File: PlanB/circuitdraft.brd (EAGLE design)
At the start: 24 x 43 mm, 23 parts, among them Q1 16 MHz

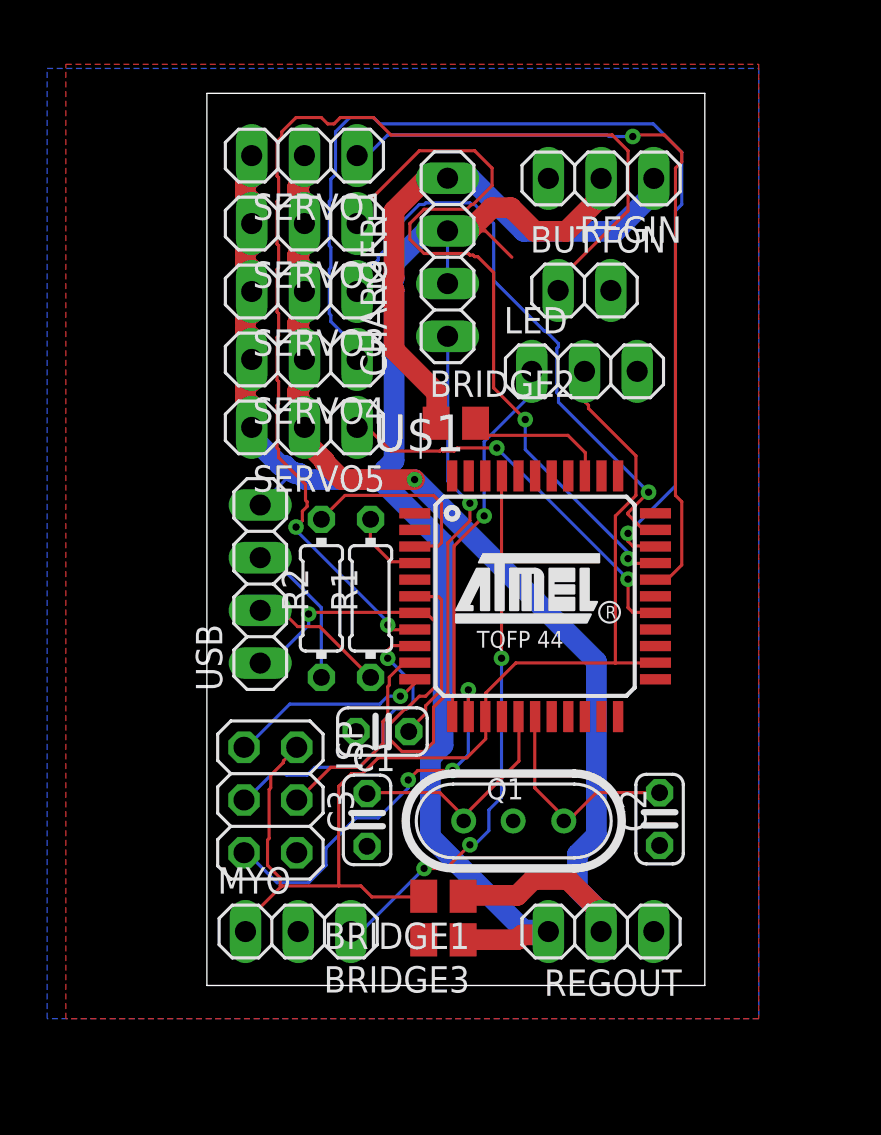
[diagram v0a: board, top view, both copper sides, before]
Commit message: more ajustments
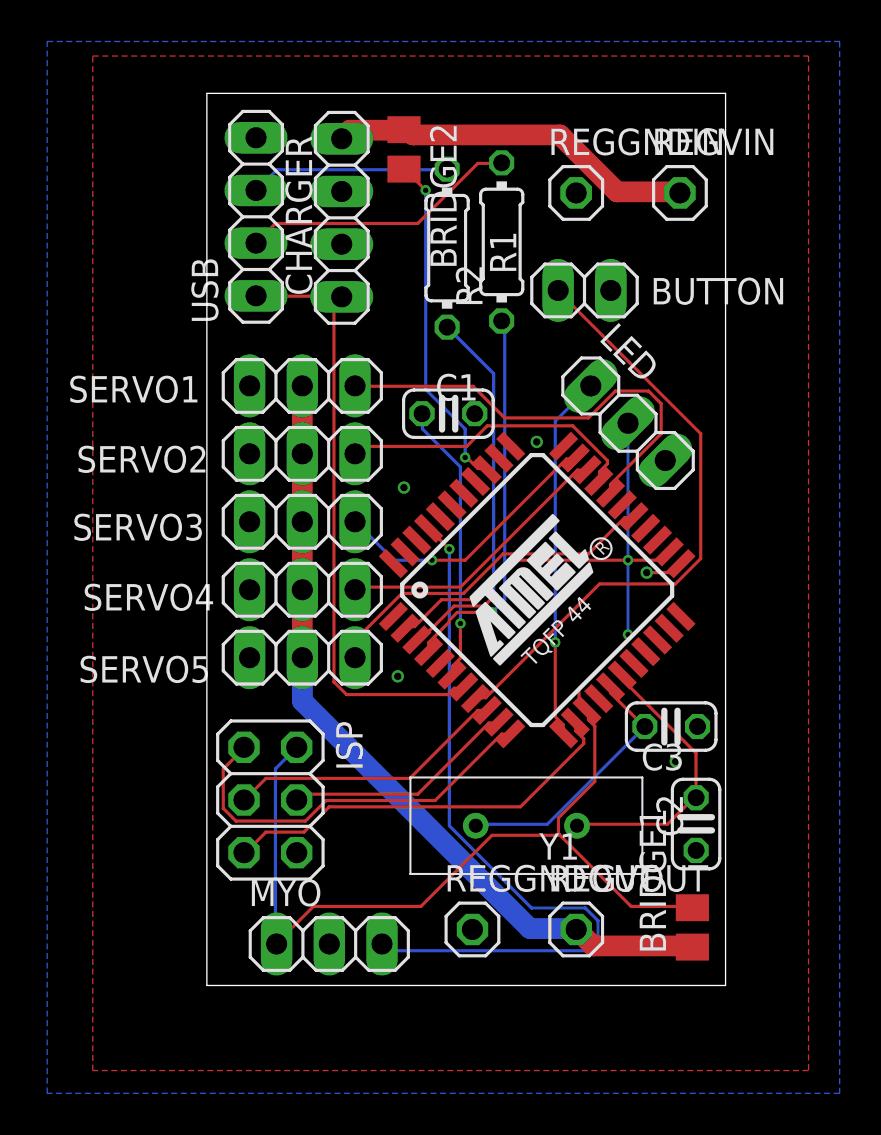
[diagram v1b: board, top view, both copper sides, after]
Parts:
- removed BRIDGE3: (no value), rcl:M0805
- removed Q1: 16 MHz, crystal:HC49U
- removed REGIN, REGOUT: (no value), pinhead:1X03
- added REGGNDIN, REGGNDOUT, REGVIN, REGVOUT: (no value), pinhead:1X01
- added Y1: CY16BPS, SamacSys_Parts:CY16BPS
- moved R1 18.3 mm to (19.2, 35.8), turned to 270 degrees
- moved R2 17.9 mm to (16.6, 35.5), turned to 270 degrees
- moved USB 17.7 mm to (7.37, 37.0)
- moved C1 15.6 mm to (16.6, 27.6), turned to 0 degrees
- moved C3 15.3 mm to (27.4, 12.5), turned to 180 degrees
- moved BRIDGE2 13.4 mm to (14.5, 40.3), turned to 270 degrees
- moved BRIDGE1 12.1 mm to (28.4, 2.80), turned to 90 degrees
- moved SERVO1 11.1 mm to (9.60, 28.9)
- moved SERVO2 11.1 mm to (9.60, 25.6)
- moved SERVO3 11.1 mm to (9.60, 22.4)
- moved SERVO4 11.1 mm to (9.60, 19.1)
- moved SERVO5 11.1 mm to (9.60, 15.8)
- moved CHARGER 5.44 mm to (11.5, 37.0)
- moved LED 3.26 mm to (25.3, 27.1), turned to 315 degrees
- moved C2 1.78 mm to (28.6, 7.78)
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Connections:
- removed net BIGGND: BRIDGE3.1, CHARGER.3, REGIN.2, REGOUT.3, SERVO1.3, SERVO2.3, SERVO3.3, SERVO4.3, SERVO5.3
- net BIGPOWER: now also REGVOUT.1; no longer REGOUT.2
- net GND: now also CHARGER.3, REGGNDIN.1, REGGNDOUT.1, SERVO1.3, SERVO2.3, SERVO3.3, SERVO4.3, SERVO5.3, U$1.15, U$1.35, U$1.43; no longer BRIDGE3.2
- net N$5: now also C2.2, U$1.17, Y1.2; no longer C3.2, Q1.1, U$1.16
- net N$6: now also C3.2, U$1.16, Y1.1; no longer C2.2, Q1.3, U$1.17
- net POWER: now also U$1.2
- net VBAT: now also REGVIN.1; no longer REGIN.1
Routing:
- net BIGGND: track 79.7 -> 0.00 mm
- net SIGNAL4: track 50.7 -> 13.6 mm, vias 1 -> 0
- net INTERRUPT: track 54.2 -> 29.4 mm, vias 2 -> 0
- net SIGNAL2: track 37.5 -> 14.6 mm, vias 2 -> 0
- net BIGPOWER: track 55.7 -> 38.9 mm, vias 1 -> 0
- net SIGNAL1: track 38.2 -> 21.5 mm, vias 1 -> 0
- net SIGNAL3: track 28.8 -> 13.4 mm
- net N$4: track 3.67 -> 18.5 mm, vias 0 -> 1
- net POWER: track 56.9 -> 69.8 mm, vias 0 -> 2
- net VBUS: track 40.0 -> 29.8 mm, vias 2 -> 0
- net MISO: track 9.74 -> 19.2 mm, vias 1 -> 0
- net N$9: track 7.01 -> 16.4 mm, vias 0 -> 2
- net N$1: track 26.0 -> 35.4 mm, vias 3 -> 1
- net VBAT: track 26.9 -> 17.7 mm
- net N$2: track 9.69 -> 18.5 mm, vias 0 -> 1
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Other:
- board size 24 x 43 mm -> 25 x 43 mm
